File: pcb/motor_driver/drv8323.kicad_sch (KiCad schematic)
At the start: 16 parts

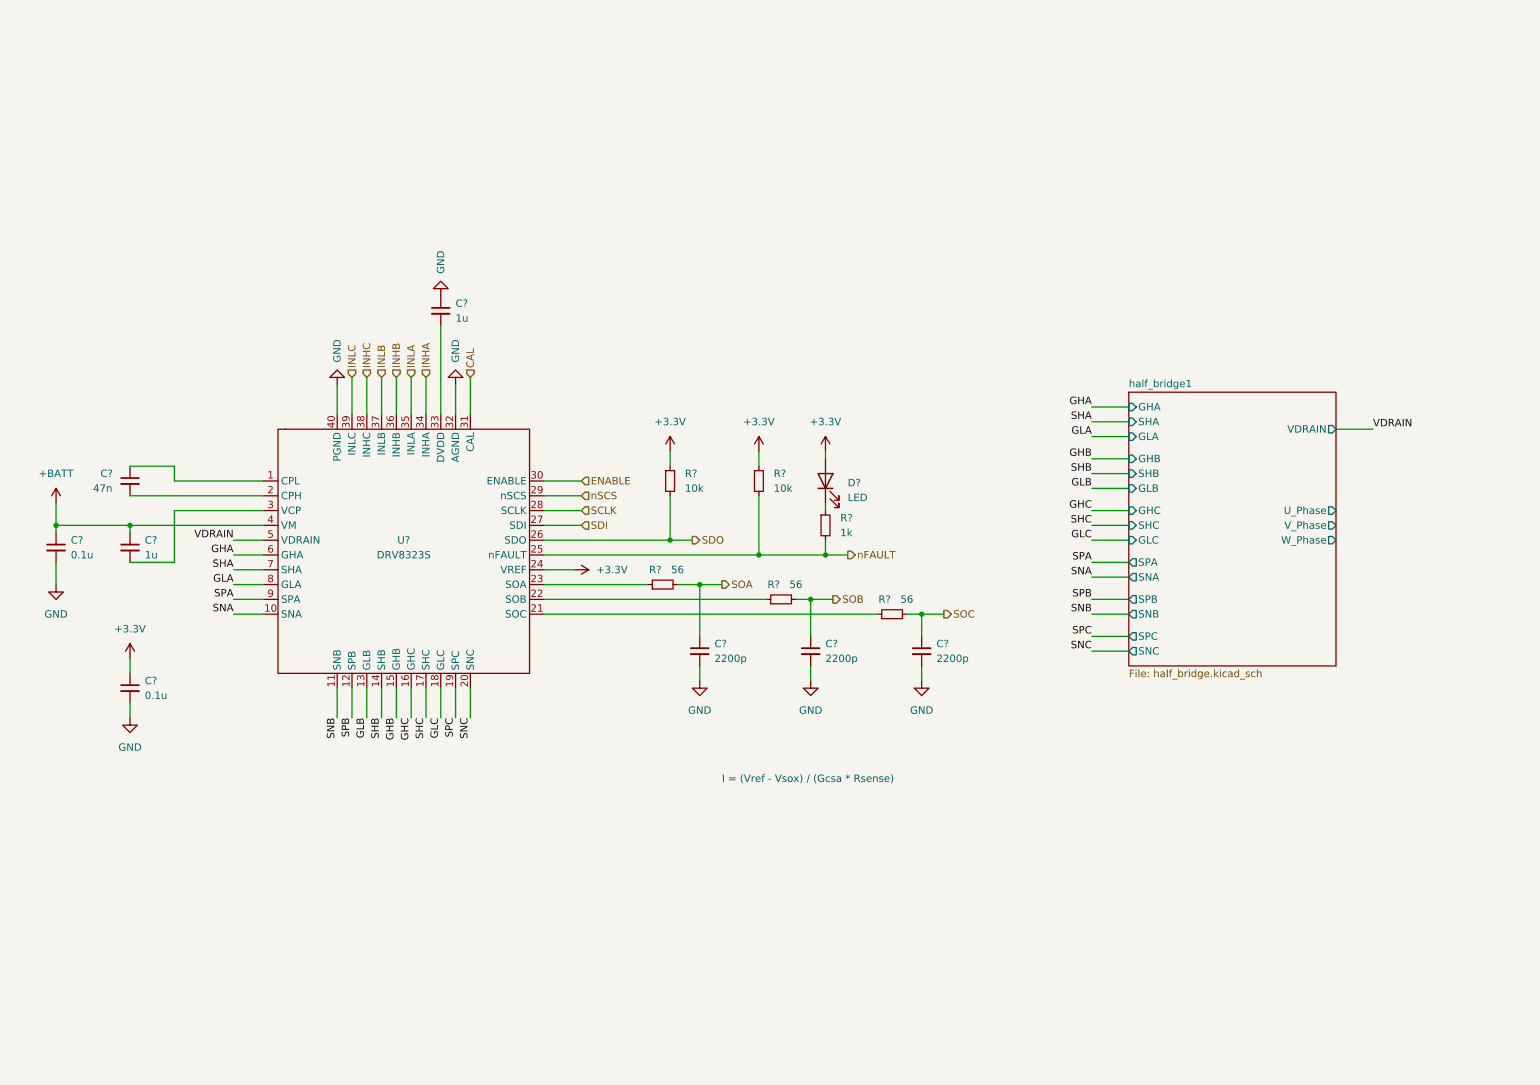
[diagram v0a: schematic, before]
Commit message: update pcb
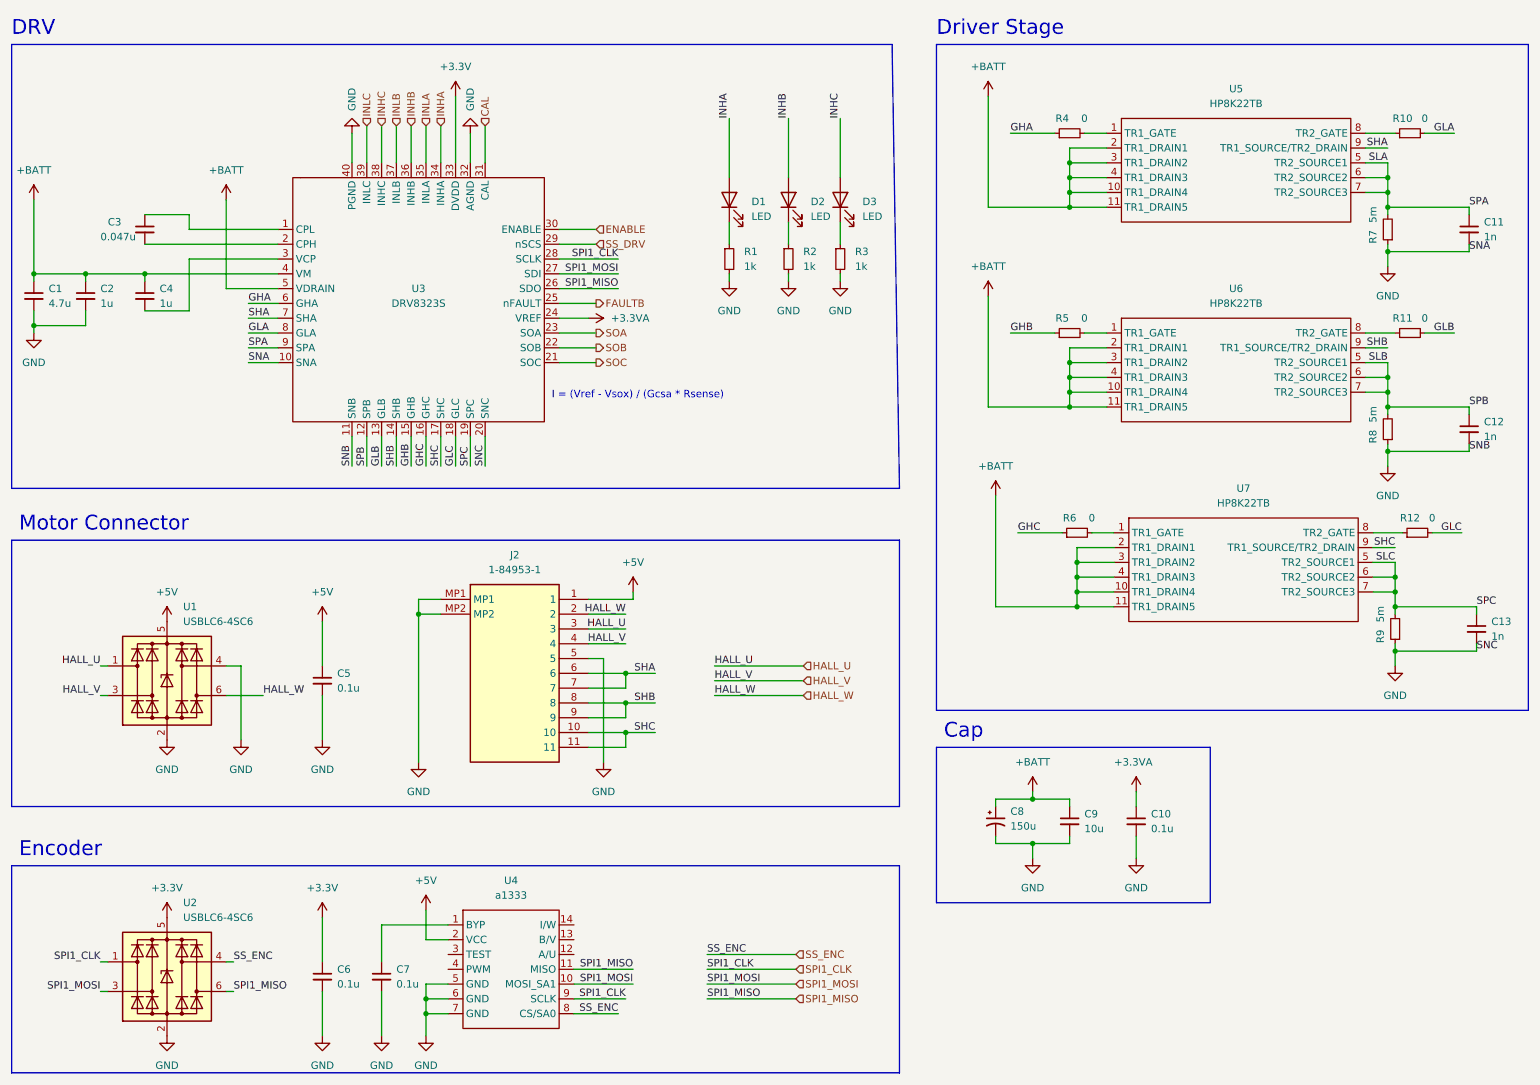
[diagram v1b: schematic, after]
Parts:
- removed C? (x2): 1u, Capacitor_SMD:C_0603_1608Metric_Pad1.08x0.95mm_HandSolder, symbol Device:C_Small
- removed C? (x2): 0.1u, Capacitor_SMD:C_0603_1608Metric_Pad1.08x0.95mm_HandSolder, symbol Device:C_Small
- removed C? (x3): 2200p, Capacitor_SMD:C_0603_1608Metric_Pad1.08x0.95mm_HandSolder, symbol Device:C_Small
- removed C?: 47n, Capacitor_SMD:C_0603_1608Metric_Pad1.08x0.95mm_HandSolder, symbol Device:C_Small
- removed D?: LED, LED_SMD:LED_0603_1608Metric_Pad1.05x0.95mm_HandSolder, symbol Device:LED
- removed R?: 1k, Resistor_SMD:R_0805_2012Metric_Pad1.20x1.40mm_HandSolder, symbol Device:R_Small
- removed R? (x3): 56, Resistor_SMD:R_0805_2012Metric_Pad1.20x1.40mm_HandSolder, symbol Device:R_Small
- removed R? (x2): 10k, Resistor_SMD:R_0603_1608Metric_Pad0.98x0.95mm_HandSolder, symbol Device:R_Small
- removed U?: DRV8323S, Package_DFN_QFN:QFN-40-1EP_6x6mm_P0.5mm_EP4.6x4.6mm_ThermalVias, symbol bldc_lib:DRV8323S
- added C1: 4.7u, Capacitor_SMD:C_0603_1608Metric_Pad1.08x0.95mm_HandSolder, symbol Device:C_Small
- added C10: 0.1u, Capacitor_SMD:C_0402_1005Metric_Pad0.74x0.62mm_HandSolder, symbol Device:C_Small
- added C11, C12, C13: 1n, Capacitor_SMD:C_0402_1005Metric_Pad0.74x0.62mm_HandSolder, symbol Device:C_Small
- added C2, C4: 1u, Capacitor_SMD:C_0603_1608Metric_Pad1.08x0.95mm_HandSolder, symbol Device:C_Small
- added C3: 0.047u, Capacitor_SMD:C_0603_1608Metric_Pad1.08x0.95mm_HandSolder, symbol Device:C_Small
- added C5, C6, C7: 0.1u, Capacitor_SMD:C_0603_1608Metric_Pad1.08x0.95mm_HandSolder, symbol Device:C_Small
- added C8: 150u, Capacitor_SMD:CP_Elec_8x10.5, symbol Device:C_Polarized_Small_US
- added C9: 10u, Capacitor_SMD:C_0603_1608Metric_Pad1.08x0.95mm_HandSolder, symbol Device:C_Small
- added D1, D2, D3: LED, LED_SMD:LED_0603_1608Metric_Pad1.05x0.95mm_HandSolder, symbol Device:LED
- added J2: 1-84953-1, bldc_lib:1-84953-1, symbol bldc_lib:1-84953-1
- added R1, R2, R3: 1k, Resistor_SMD:R_0402_1005Metric_Pad0.72x0.64mm_HandSolder, symbol Device:R_Small
- added R10, R11, R12, R4, R5, R6: 0, Resistor_SMD:R_0805_2012Metric_Pad1.20x1.40mm_HandSolder, symbol Device:R_Small
- added R7, R8, R9: 5m, Resistor_SMD:R_2010_5025Metric_Pad1.40x2.65mm_HandSolder, symbol Device:R_Small
- added U1, U2: USBLC6-4SC6, Package_TO_SOT_SMD:SOT-23-6, symbol Power_Protection:USBLC6-4SC6
- added U3: DRV8323S, Package_DFN_QFN:QFN-40-1EP_6x6mm_P0.5mm_EP4.6x4.6mm_ThermalVias, symbol bldc_lib:DRV8323S
- added U4: a1333, Package_SO:HTSSOP-14-1EP_4.4x5mm_P0.65mm_EP3.4x5mm_Mask3x3.1mm, symbol bldc_lib:a1333
- added U5, U6, U7: HP8K22TB, bldc_lib:HP8K24TB, symbol bldc_lib:HP8K22TB
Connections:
- net +3.3V: now also C6.1, U2.5 (VBUS), U3.33 (DVDD)
- net +BATT: now also C1.1, C2.1, C4.1, C8.1, C9.1, U3.4 (VM), U3.5 (VDRAIN), U5.10 (TR1_DRAIN4), U5.11 (TR1_DRAIN5), U5.2 (TR1_DRAIN1), U5.3 (TR1_DRAIN2), U5.4 (TR1_DRAIN3), U6.10 (TR1_DRAIN4), U6.11 (TR1_DRAIN5), U6.2 (TR1_DRAIN1), U6.3 (TR1_DRAIN2), U6.4 (TR1_DRAIN3), U7.10 (TR1_DRAIN4), U7.11 (TR1_DRAIN5), U7.2 (TR1_DRAIN1), U7.3 (TR1_DRAIN2), U7.4 (TR1_DRAIN3)
- net CAL: now also U3.31 (CAL)
- net ENABLE: now also U3.30 (ENABLE)
- net GHA: now also R4.1, U3.6 (GHA)
- net GHB: now also R5.1, U3.15 (GHB)
- net GHC: now also R6.1, U3.16 (GHC)
- net GLA: now also R10.2, U3.8 (GLA)
- net GLB: now also R11.2, U3.13 (GLB)
- net GLC: now also R12.2, U3.18 (GLC)
- net GND: now also C1.2, C10.2, C11.2, C12.2, C13.2, C2.2, C5.2, C6.2, C7.2, C8.2, C9.2, J2.5, J2.MP1, J2.MP2, R1.2, R2.2, R3.2, R7.1, R8.1, R9.1, U1.2 (GND), U1.4 (I/O3), U2.2 (GND), U3.10 (SNA), U3.11 (SNB), U3.20 (SNC), U3.32 (AGND), U3.40 (PGND), U4.5 (GND), U4.6 (GND), U4.7 (GND)
- net INHA: now also D1.2 (A), U3.34 (INHA)
- net INHB: now also D2.2 (A), U3.36 (INHB)
- net INHC: now also D3.2 (A), U3.38 (INHC)
- net INLA: now also U3.35 (INLA)
- net INLB: now also U3.37 (INLB)
- net INLC: now also U3.39 (INLC)
- net SHA: now also J2.6, J2.7, U3.7 (SHA), U5.9 (TR1_SOURCE/TR2_DRAIN)
- net SHB: now also J2.8, J2.9, U3.14 (SHB), U6.9 (TR1_SOURCE/TR2_DRAIN)
- net SHC: now also J2.10, J2.11, U3.17 (SHC), U7.9 (TR1_SOURCE/TR2_DRAIN)
- net SOA: now also U3.23 (SOA)
- net SOB: now also U3.22 (SOB)
- net SOC: now also U3.21 (SOC)
- new net: R11.1, U6.8 (TR2_GATE)
- new net: C7.1, U4.1 (BYP)
- new net: D1.1 (K), R1.1
- new net: R5.2, U6.1 (TR1_GATE)
- new net: R12.1, U7.8 (TR2_GATE)
- new net: R4.2, U5.1 (TR1_GATE)
- new net: D2.1 (K), R2.1
- new net: C4.2, U3.3 (VCP)
- new net: R6.2, U7.1 (TR1_GATE)
- new net: C3.1, U3.1 (CPL)
- new net: C3.2, U3.2 (CPH)
- new net: D3.1 (K), R3.1
- new net: R10.1, U5.8 (TR2_GATE)
- new net +3.3VA: C10.1, U3.24 (VREF)
- new net +5V: C5.1, J2.1, U1.5 (VBUS), U4.2 (VCC)
- new net FAULTB: U3.25 (nFAULT)
- new net HALL_U: J2.3, U1.1 (I/O1)
- new net HALL_V: J2.4, U1.3 (I/O2)
- new net HALL_W: J2.2, U1.6 (I/O4)
- new net SLA: C11.1, R7.2, U3.9 (SPA), U5.5 (TR2_SOURCE1), U5.6 (TR2_SOURCE2), U5.7 (TR2_SOURCE3)
- new net SLB: C12.1, R8.2, U3.12 (SPB), U6.5 (TR2_SOURCE1), U6.6 (TR2_SOURCE2), U6.7 (TR2_SOURCE3)
- new net SLC: C13.1, R9.2, U3.19 (SPC), U7.5 (TR2_SOURCE1), U7.6 (TR2_SOURCE2), U7.7 (TR2_SOURCE3)
- new net SPI1_CLK: U2.1 (I/O1), U3.28 (SCLK), U4.9 (SCLK)
- new net SPI1_MISO: U2.6 (I/O4), U3.26 (SDO), U4.11 (MISO)
- new net SPI1_MOSI: U2.3 (I/O2), U3.27 (SDI), U4.10 (MOSI_SA1)
- new net SS_DRV: U3.29 (nSCS)
- new net SS_ENC: U2.4 (I/O3), U4.8 (CS/SA0)
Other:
- removed sheet half_bridge1
- note added: "Cap"
- note added: "DRV"
- note added: "Driver Stage"
- note added: "Encoder"
- note added: "Motor Connector"
